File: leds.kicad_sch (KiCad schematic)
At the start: 4 parts

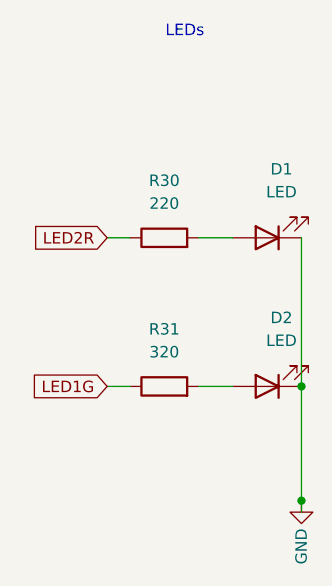
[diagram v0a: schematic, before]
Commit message: Solve all warnings
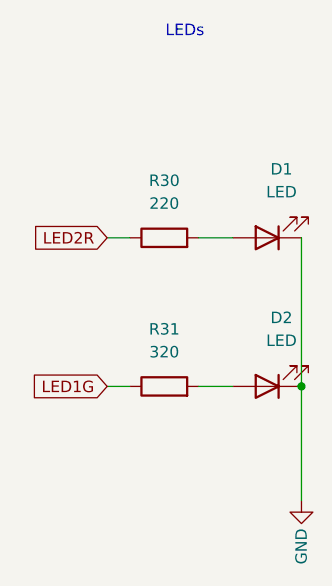
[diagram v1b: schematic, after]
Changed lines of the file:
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@@
-	)
-	(junction
-		(at 69.85 78.74)
-		(diameter 0)
-		(color 0 0 0 0)
 	)
 	(junction
@@
 	(wire
 		(pts
-			(xy 69.85 49.53) (xy 69.85 66.04)
+			(xy 69.85 66.04) (xy 69.85 78.74)
 		)
 		(stroke
@@
 	(wire
 		(pts
-			(xy 69.85 78.74) (xy 69.85 80.01)
+			(xy 69.85 49.53) (xy 69.85 66.04)
 		)
 		(stroke
-			(width 0)
-			(type default)
-		)
-	)
-	(wire
-		(pts
-			(xy 69.85 66.04) (xy 69.85 78.74)
-		)
-		(stroke
